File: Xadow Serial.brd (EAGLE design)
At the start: 28.1 x 20.3 mm, 28 parts, among them J1 CONNECTOR-HEADER-8P-3461050P1, J2 12p 0.5mm bottom contact, J3 12p 0.5mm bottom contact, J4 12p 0.5mm bottom contact, U1 SC16IS750, U2 BSS138PS, X1 CTS_32X25_SMD

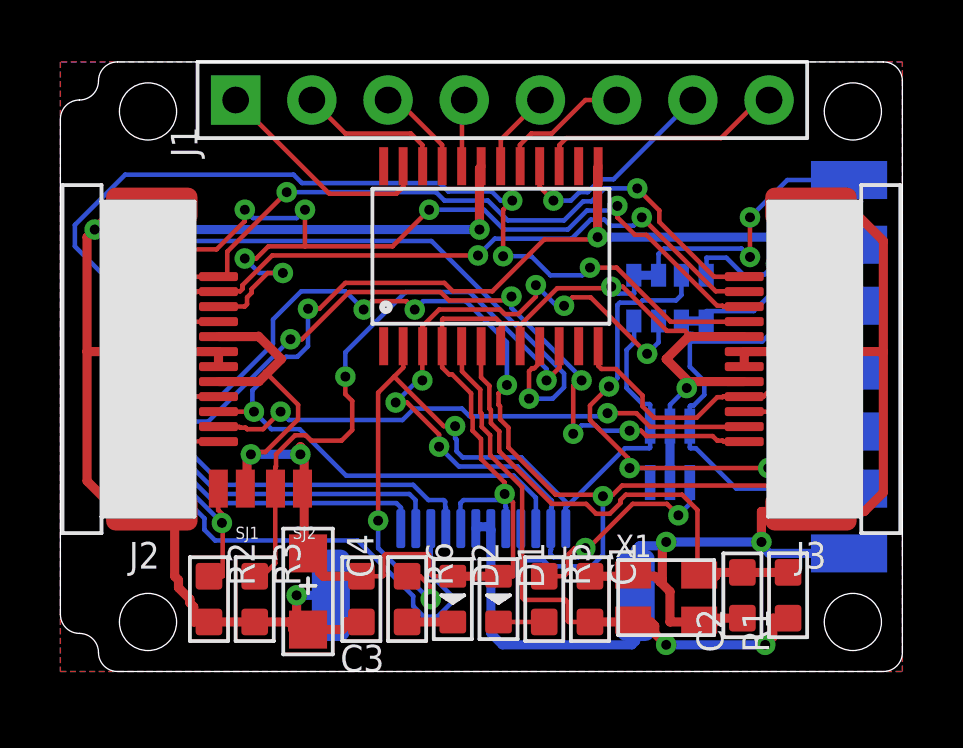
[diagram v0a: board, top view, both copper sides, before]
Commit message: Fixed up labels
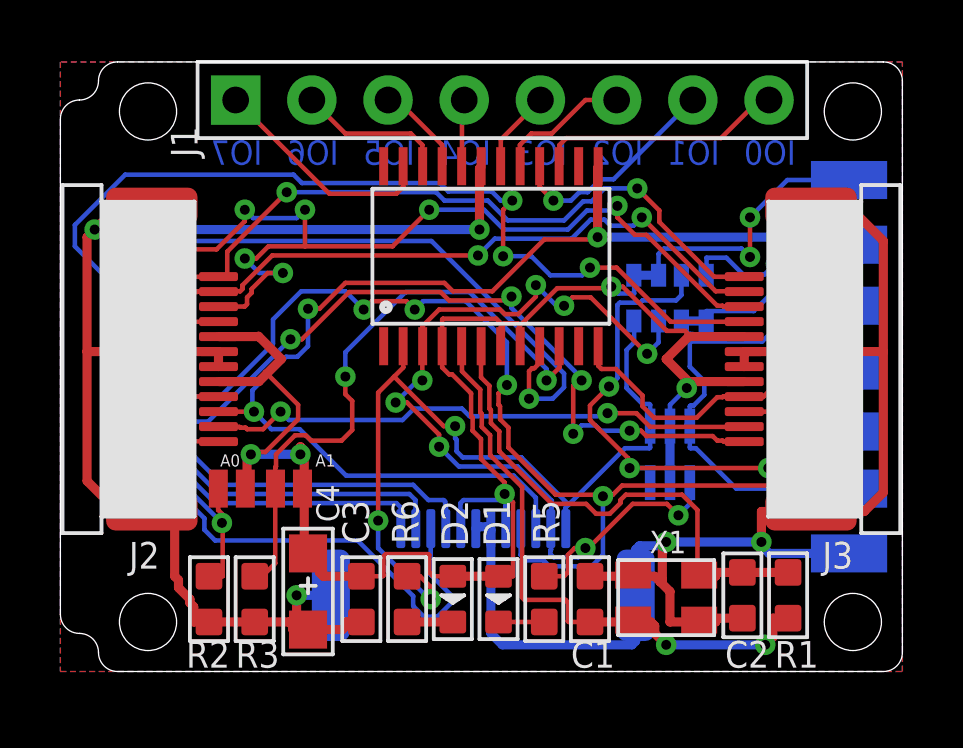
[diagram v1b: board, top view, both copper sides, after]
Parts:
- renumbered SJ1 to A0, SJ2 to A1
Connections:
- net N$11 renamed IO4
- net N$12 renamed IO5
- net N$13 renamed IO6
- net N$14 renamed IO7
- net N$6 renamed IO0
- net N$7 renamed IO1
- net N$8 renamed IO2
- net N$9 renamed IO3
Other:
- board text added: "IO0"
- board text added: "IO1"
- board text added: "IO2"
- board text added: "IO3"
- board text added: "IO4"
- board text added: "IO5"
- board text added: "IO6"
- board text added: "IO7"
